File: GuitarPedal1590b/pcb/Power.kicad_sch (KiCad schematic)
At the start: 10 parts, among them U1 LD1117S50TR_SOT223, U2 PDS1-S5-S5-M

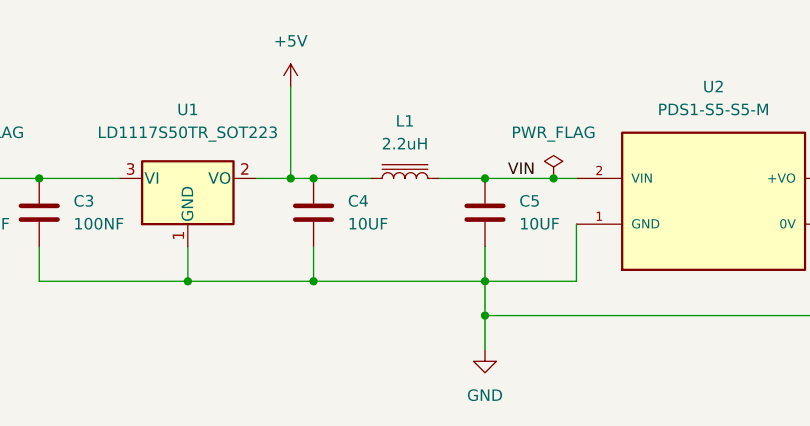
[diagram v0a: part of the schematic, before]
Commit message: Updated project to KiCad 7
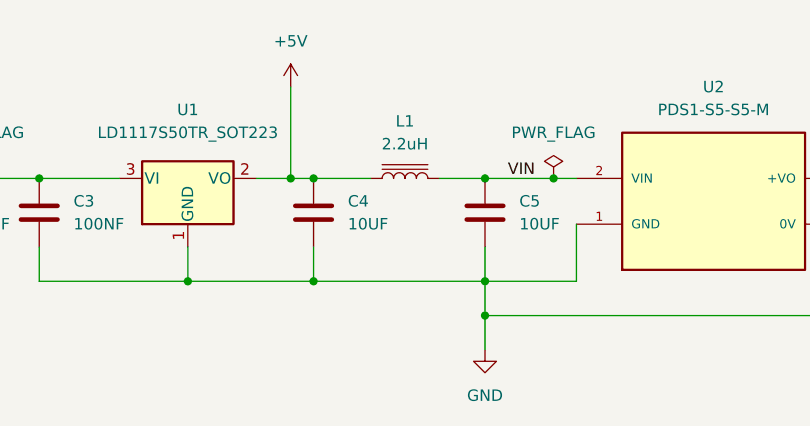
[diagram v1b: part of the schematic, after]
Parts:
- U1: footprint Package_TO_SOT_SMD:TO-252-2 -> Package_TO_SOT_SMD:TO-252-3_TabPin2

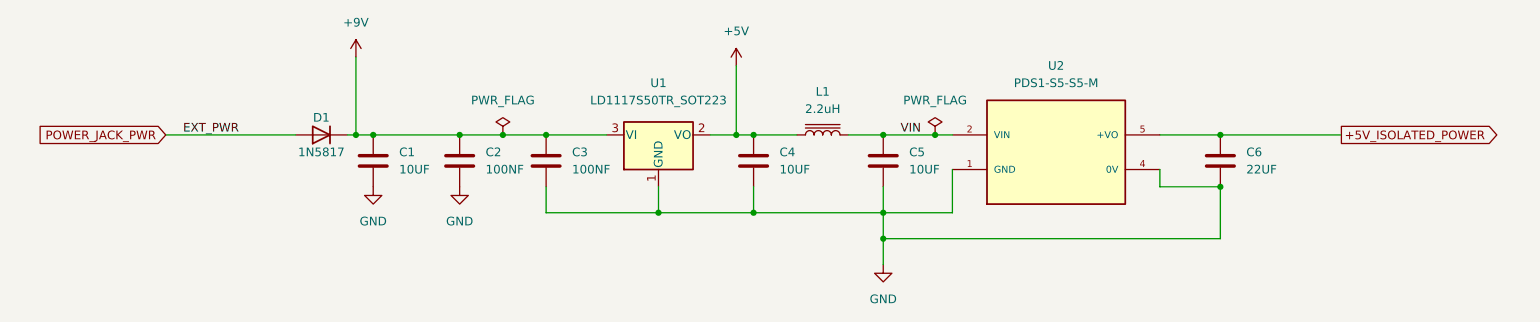
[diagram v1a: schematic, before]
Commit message: KiCad 7 fixes
Had to update some footprints and symbols to address issues related to ugprading to KiCad 7.0
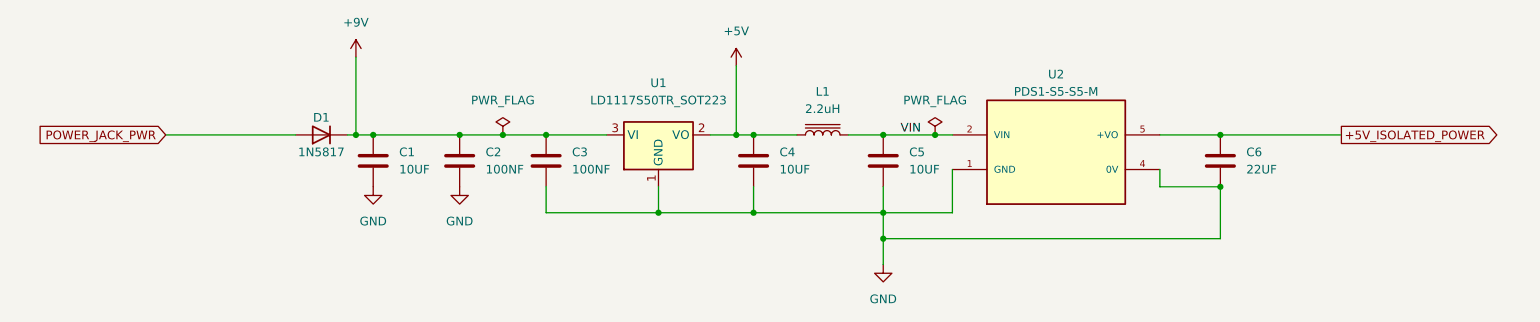
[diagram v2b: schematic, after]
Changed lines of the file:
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@@
-    (effects (font (size 1.27 1.27)) (justify left bottom))
-  )
-  (label "EXT_PWR" (at 48.26 100.33 0) (fields_autoplaced)
     (effects (font (size 1.27 1.27)) (justify left bottom))
   )
@@
       (effects (font (size 1.27 1.27)) hide)
     )
+    (property "Sim.Device" "D" (at 68.58 100.33 0)
+      (effects (font (size 1.27 1.27)) hide)
+    )
+    (property "Sim.Pins" "1=K 2=A" (at 68.58 100.33 0)
+      (effects (font (size 1.27 1.27)) hide)
+    )
     (pin "1")
     (pin "2")
@@
   (symbol (lib_id "PDS1-S5-S5-M:PDS1-S5-S5-M") (at 176.53 102.87 0) (unit 1)
     (in_bom yes) (on_board yes) (dnp no) (fields_autoplaced)
-    (property "Reference" "U2" (at 176.53 90.17 0)
-      (effects (font (size 1.27 1.27)))
-    )
-    (property "Value" "PDS1-S5-S5-M" (at 176.53 92.71 0)
-      (effects (font (size 1.27 1.27)))
-    )
+    (property "Reference" "U2" (at 176.53 91.44 0)
+      (effects (font (size 1.27 1.27)))
+    )
+    (property "Value" "PDS1-S5-S5-M" (at 176.53 93.98 0)
+      (effects (font (size 1.27 1.27)))
+    )
